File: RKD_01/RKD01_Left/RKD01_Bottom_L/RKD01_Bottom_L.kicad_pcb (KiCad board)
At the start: 2 copper layers, 164.3 x 126.2 mm, 8 parts

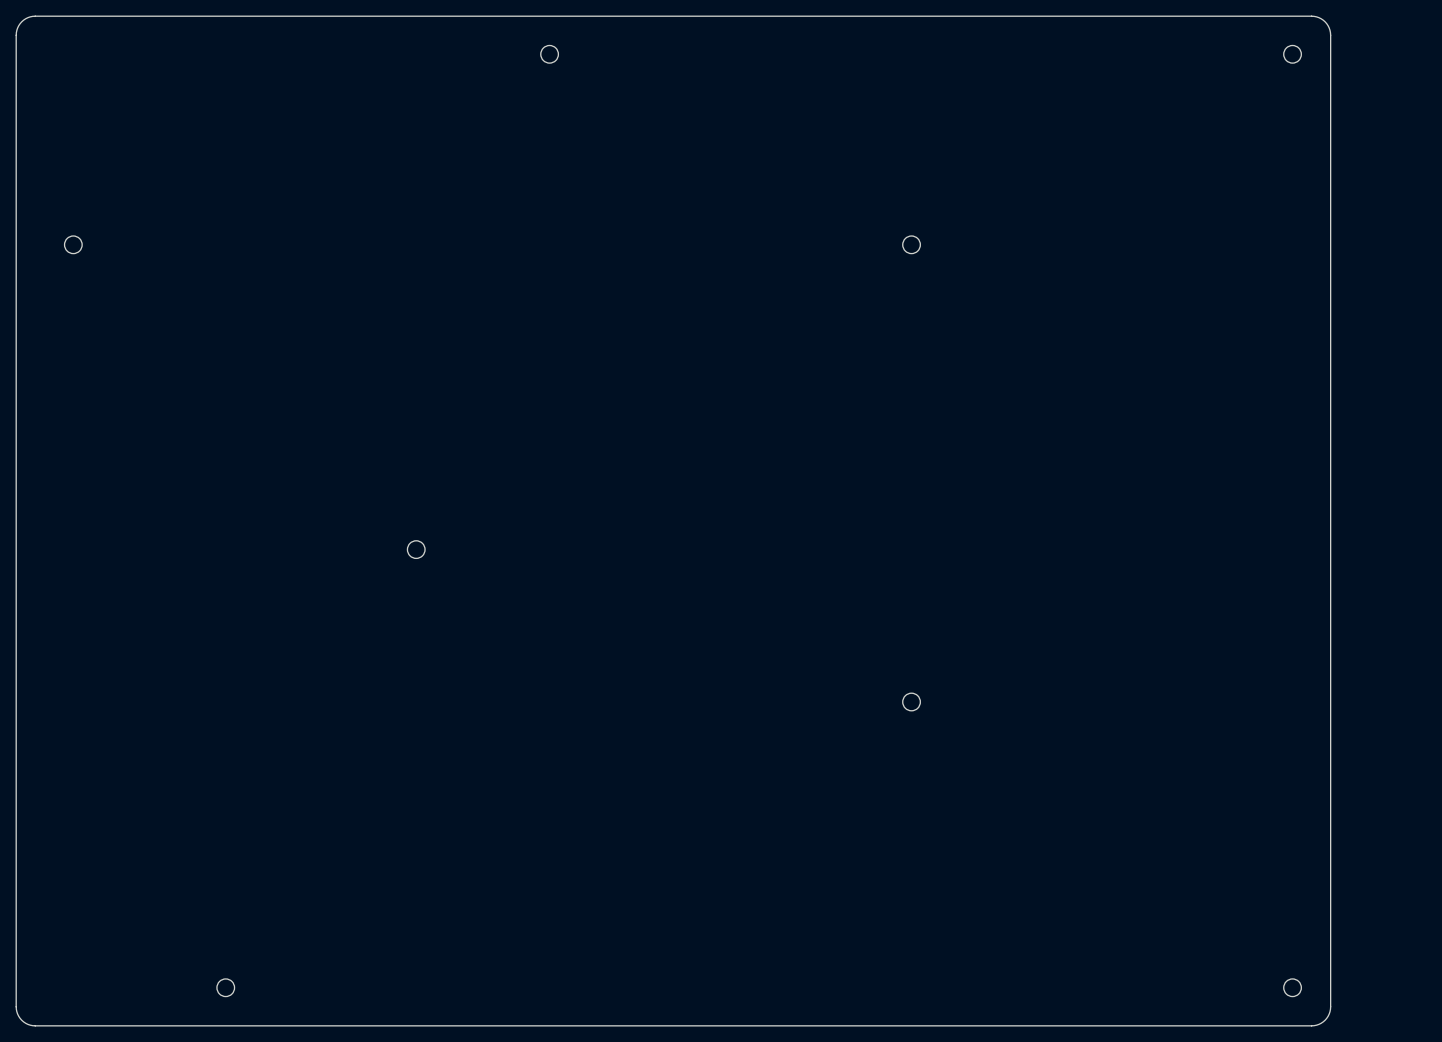
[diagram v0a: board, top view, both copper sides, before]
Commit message: 寸法を見直し
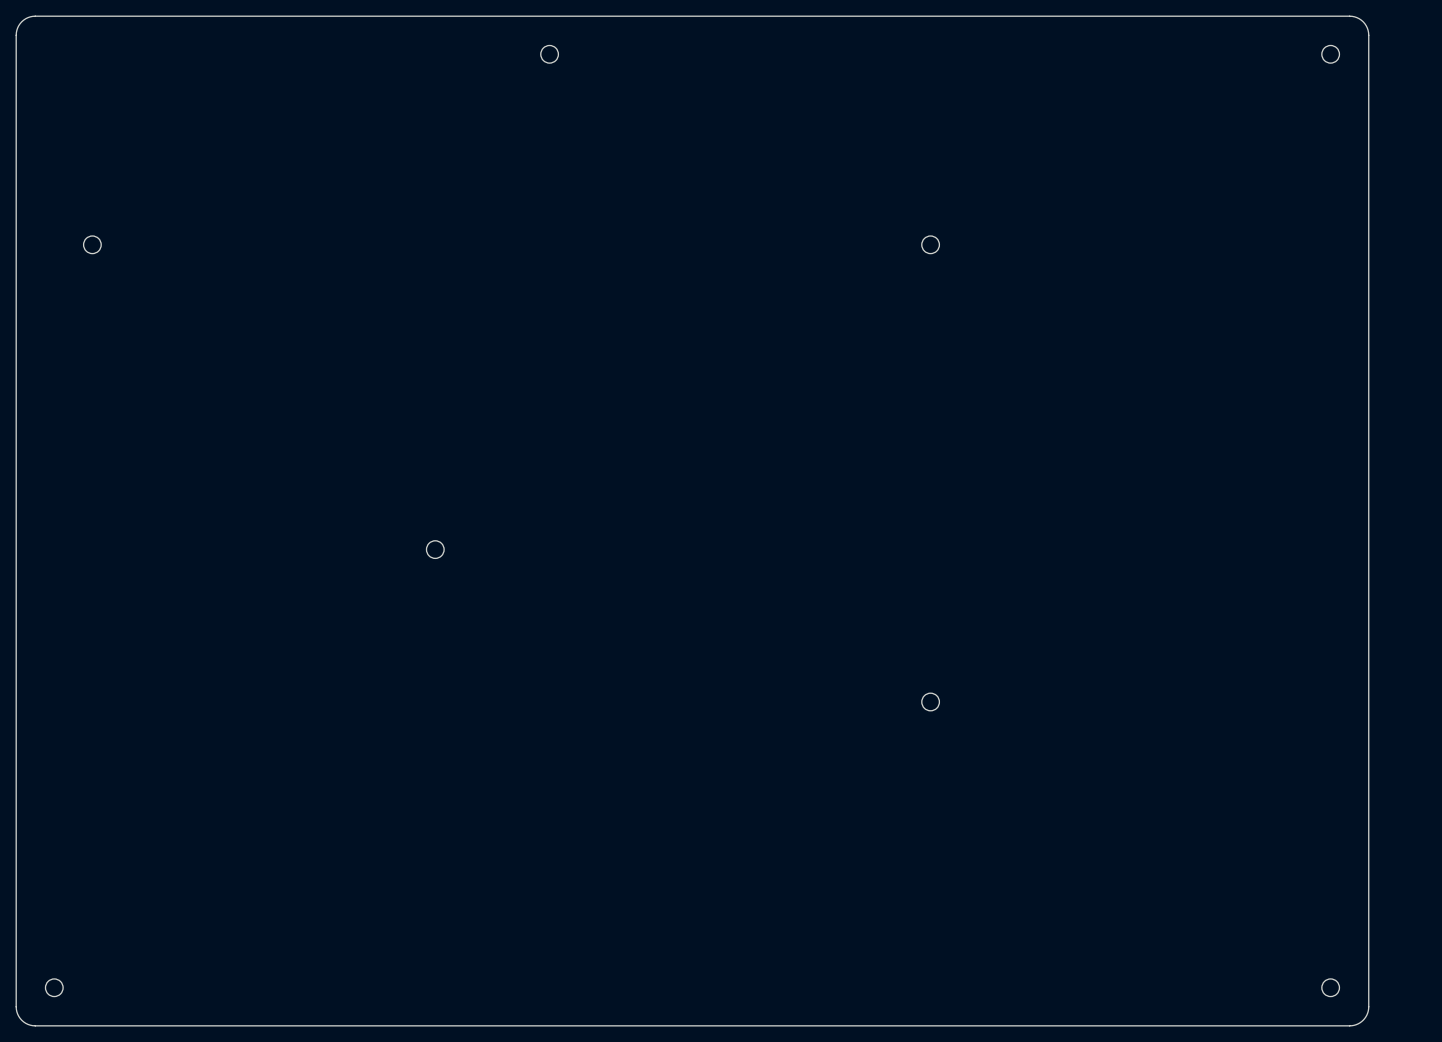
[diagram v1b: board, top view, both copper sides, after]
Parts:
- M1, M2, M3, M4, M5, M6, M7, M8: renamed from Ref**; value Val** -> Mark
- moved M7 21.4 mm to (26.2, 140.5)
- moved M8 4.76 mm to (185.7, 140.5)
- moved M2 4.76 mm to (185.7, 23.8)
- moved M4 2.38 mm to (135.7, 47.6)
- moved M6 2.38 mm to (135.7, 104.8)
- moved M3 2.38 mm to (31.0, 47.6)
- moved M5 2.38 mm to (73.8, 85.7)
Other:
- board size 164.3 x 126.2 mm -> 169.1 x 126.2 mm
- board text added: "RKD01_Left v1.0"
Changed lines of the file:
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@@
 			(drillshape 0)
 			(scaleselection 1)
-			(outputdirectory "../../../../Order/20241231/RKD01/Bottom_L/")
+			(outputdirectory "../../../../Order/20241231/RKD01/Assemble_L/")
 		)
 	)
@@
 	(footprint "kbd_Hole:m2_Screw_Hole"
 		(layer "F.Cu")
-		(at 133.35 104.775)
+		(at 135.7313 104.775)
 		(descr "Mounting Hole 2.2mm, no annular, M2")
 		(tags "mounting hole 2.2mm no annular m2")
-		(property "Reference" "Ref**"
+		(property "Reference" "M6"
 			(at 0 -3.2 0)
 			(layer "F.Fab")
@@
 			)
 		)
-		(property "Value" "Val**"
+		(property "Value" "Mark"
 			(at 0 3.2 0)
 			(layer "F.Fab")
@@
 			)
 		)
+		(sheetname "ルート")
+		(sheetfile "RKD01_Assemble_L.kicad_sch")
 		(attr exclude_from_pos_files exclude_from_bom)
 		(fp_circle
@@
 	(footprint "kbd_Hole:m2_Screw_Hole"
 		(layer "F.Cu")
-		(at 71.4375 85.725)
+		(at 73.8188 85.725)
 		(descr "Mounting Hole 2.2mm, no annular, M2")
 		(tags "mounting hole 2.2mm no annular m2")
-		(property "Reference" "Ref**"
+		(property "Reference" "M5"
 			(at 0 -3.2 0)
 			(layer "F.Fab")
@@
 			)
 		)
-		(property "Value" "Val**"
+		(property "Value" "Mark"
 			(at 0 3.2 0)
 			(layer "F.Fab")
@@
 			)
 		)
+		(sheetname "ルート")
+		(sheetfile "RKD01_Assemble_L.kicad_sch")
 		(attr exclude_from_pos_files exclude_from_bom)
 		(fp_circle
@@
 	(footprint "kbd_Hole:m2_Screw_Hole"
 		(layer "F.Cu")
-		(at 180.975 23.8125)
+		(at 185.7375 23.8125)
 		(descr "Mounting Hole 2.2mm, no annular, M2")
 		(tags "mounting hole 2.2mm no annular m2")
-		(property "Reference" "Ref**"
+		(property "Reference" "M2"
 			(at 0 -3.2 0)
 			(layer "F.Fab")
@@
 			)
 		)
-		(property "Value" "Val**"
+		(property "Value" "Mark"
 			(at 0 3.2 0)
 			(layer "F.Fab")
@@
 			)
 		)
+		(sheetname "ルート")
+		(sheetfile "RKD01_Assemble_L.kicad_sch")
 		(attr exclude_from_pos_files exclude_from_bom)
 		(fp_circle
@@
 	(footprint "kbd_Hole:m2_Screw_Hole"
 		(layer "F.Cu")
-		(at 180.975 140.49375)
+		(at 185.7375 140.4937)
 		(descr "Mounting Hole 2.2mm, no annular, M2")
 		(tags "mounting hole 2.2mm no annular m2")
-		(property "Reference" "Ref**"
+		(property "Reference" "M8"
 			(at 0 -3.2 0)
 			(layer "F.Fab")
@@
 			)
 		)
-		(property "Value" "Val**"
+		(property "Value" "Mark"
 			(at 0 3.2 0)
 			(layer "F.Fab")
@@
 			)
 		)
+		(sheetname "ルート")
+		(sheetfile "RKD01_Assemble_L.kicad_sch")
 		(attr exclude_from_pos_files exclude_from_bom)
 		(fp_circle
@@
 	(footprint "kbd_Hole:m2_Screw_Hole"
 		(layer "F.Cu")
-		(at 47.625 140.49375)
+		(at 26.1938 140.4937)
 		(descr "Mounting Hole 2.2mm, no annular, M2")
 		(tags "mounting hole 2.2mm no annular m2")
-		(property "Reference" "Ref**"
+		(property "Reference" "M7"
 			(at 0 -3.2 0)
 			(layer "F.Fab")
@@
 			)
 		)
-		(property "Value" "Val**"
+		(property "Value" "Mark"
 			(at 0 3.2 0)
 			(layer "F.Fab")
@@
 			)
 		)
+		(sheetname "ルート")
+		(sheetfile "RKD01_Assemble_L.kicad_sch")
 		(attr exclude_from_pos_files exclude_from_bom)
 		(fp_circle
@@
 	(footprint "kbd_Hole:m2_Screw_Hole"
 		(layer "F.Cu")
-		(at 88.10625 23.8125)
+		(at 88.1063 23.8125)
 		(descr "Mounting Hole 2.2mm, no annular, M2")
 		(tags "mounting hole 2.2mm no annular m2")
-		(property "Reference" "Ref**"
+		(property "Reference" "M1"
 			(at 0 -3.2 0)
 			(layer "F.Fab")
@@
 			)
 		)
-		(property "Value" "Val**"
+		(property "Value" "Mark"
 			(at 0 3.2 0)
 			(layer "F.Fab")
@@
 			)
 		)
+		(sheetname "ルート")
+		(sheetfile "RKD01_Assemble_L.kicad_sch")
 		(attr exclude_from_pos_files exclude_from_bom)
 		(fp_circle
@@
 	(footprint "kbd_Hole:m2_Screw_Hole"
 		(layer "F.Cu")
-		(at 133.35 47.625)
+		(at 135.7313 47.625)
 		(descr "Mounting Hole 2.2mm, no annular, M2")
 		(tags "mounting hole 2.2mm no annular m2")
-		(property "Reference" "Ref**"
+		(property "Reference" "M4"
 			(at 0 -3.2 0)
 			(layer "F.Fab")
@@
 			)
 		)
-		(property "Value" "Val**"
+		(property "Value" "Mark"
 			(at 0 3.2 0)
 			(layer "F.Fab")
@@
 			)
 		)
+		(sheetname "ルート")
+		(sheetfile "RKD01_Assemble_L.kicad_sch")
 		(attr exclude_from_pos_files exclude_from_bom)
 		(fp_circle
@@
 	(footprint "kbd_Hole:m2_Screw_Hole"
 		(layer "F.Cu")
-		(at 28.575 47.625)
+		(at 30.9563 47.625)
 		(descr "Mounting Hole 2.2mm, no annular, M2")
 		(tags "mounting hole 2.2mm no annular m2")
-		(property "Reference" "Ref**"
+		(property "Reference" "M3"
 			(at 0 -3.2 0)
 			(layer "F.Fab")
@@
 			)
 		)
-		(property "Value" "Val**"
+		(property "Value" "Mark"
 			(at 0 3.2 0)
 			(layer "F.Fab")
@@
 			)
 		)
+		(sheetname "ルート")
+		(sheetfile "RKD01_Assemble_L.kicad_sch")
 		(attr exclude_from_pos_files exclude_from_bom)
 		(fp_circle
@@
 	)
 	(gr_arc
-		(start 183.35625 19.05)
-		(mid 185.040048 19.747452)
-		(end 185.7375 21.43125)
+		(start 188.1188 19.04995)
+		(mid 189.802583 19.747417)
+		(end 190.50005 21.4312)
 		(stroke
 			(width 0.05)
@@
 	)
 	(gr_line
-		(start 183.35625 19.05)
+		(start 188.1188 19.04995)
 		(end 23.8125 19.05)
 		(stroke
@@
 	)
 	(gr_arc
-		(start 21.43125 21.43125)
-		(mid 22.128702 19.747452)
-		(end 23.8125 19.05)
+		(start 21.43125 21.4313)
+		(mid 22.128702 19.747502)
+		(end 23.8125 19.05005)
 		(stroke
 			(width 0.05)
@@
 	)
 	(gr_arc
-		(start 185.7375 142.875)
-		(mid 185.040048 144.558798)
-		(end 183.35625 145.25625)
+		(start 190.50005 142.875)
+		(mid 189.802601 144.558816)
+		(end 188.1188 145.25625)
 		(stroke
 			(width 0.05)
@@
 	(gr_line
 		(start 23.8125 145.25625)
-		(end 183.35625 145.25625)
+		(end 188.1188 145.25625)
 		(stroke
 			(width 0.05)
@@
 	)
 	(gr_line
-		(start 185.7375 142.875)
-		(end 185.7375 21.43125)
+		(start 190.5 142.875)
+		(end 190.5 21.43125)
 		(stroke
 			(width 0.05)
@@
 		(layer "Edge.Cuts")
 	)
+	(gr_text "RKD01_Left v1.0"
+		(at 176.2125 23.8125 0)
+		(layer "B.SilkS")
+		(effects
+			(font
+				(size 1 1)
+				(thickness 0.1)
+			)
+			(justify left bottom mirror)
+		)
+	)
 )

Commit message: デザイン見直し
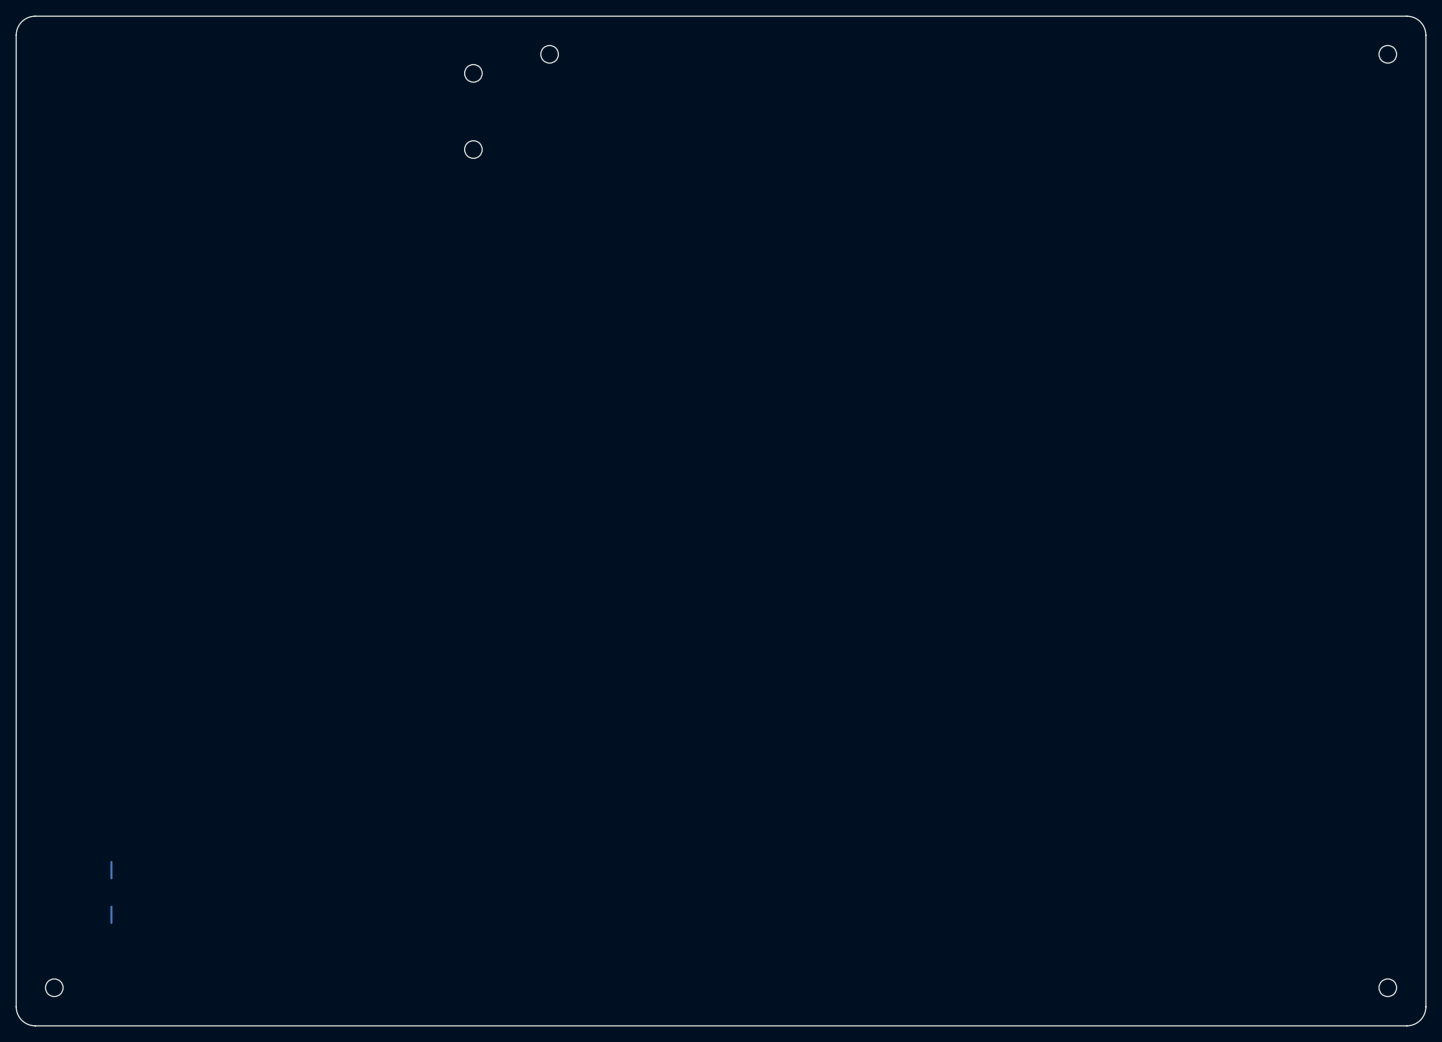
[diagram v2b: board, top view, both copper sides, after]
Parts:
- removed M7, M8: Mark, kbd_Hole:m2_Screw_Hole
- moved M4 109.0 mm to (192.9, 140.5)
- moved M3 93.0 mm to (26.2, 140.5)
- moved M6 89.6 mm to (78.6, 35.7)
- moved M5 59.7 mm to (78.6, 26.2)
- moved M2 7.14 mm to (192.9, 23.8)
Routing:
- net Row4: track 0.00 -> 2.03 mm
- net Net-(D5-A): track 0.00 -> 2.03 mm
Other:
- board size 169.1 x 126.2 mm -> 176.2 x 126.2 mm
